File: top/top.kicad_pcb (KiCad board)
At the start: 4 copper layers, 28.3 x 40 mm, 22 parts, among them P1 CONN_10, P2 CONN_5, U1 IQS572, U4 ESD

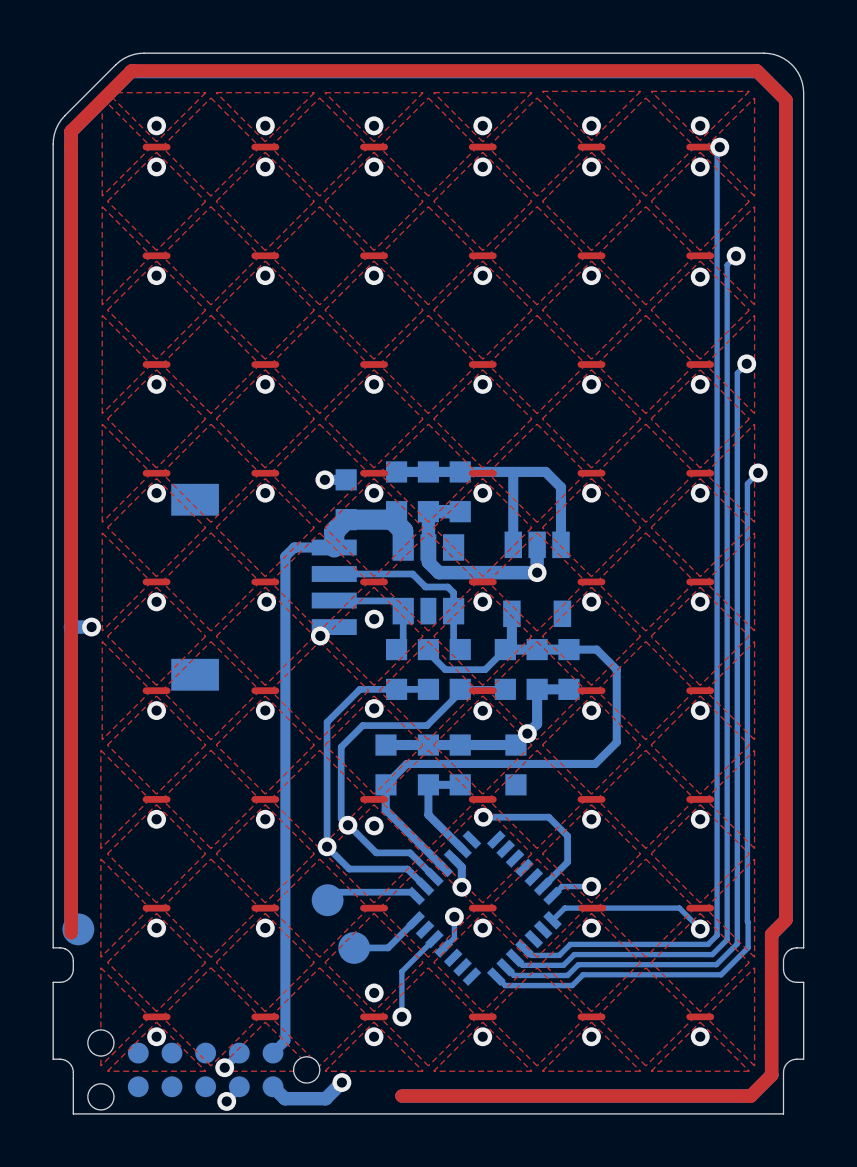
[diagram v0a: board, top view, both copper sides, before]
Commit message: First final modified board.
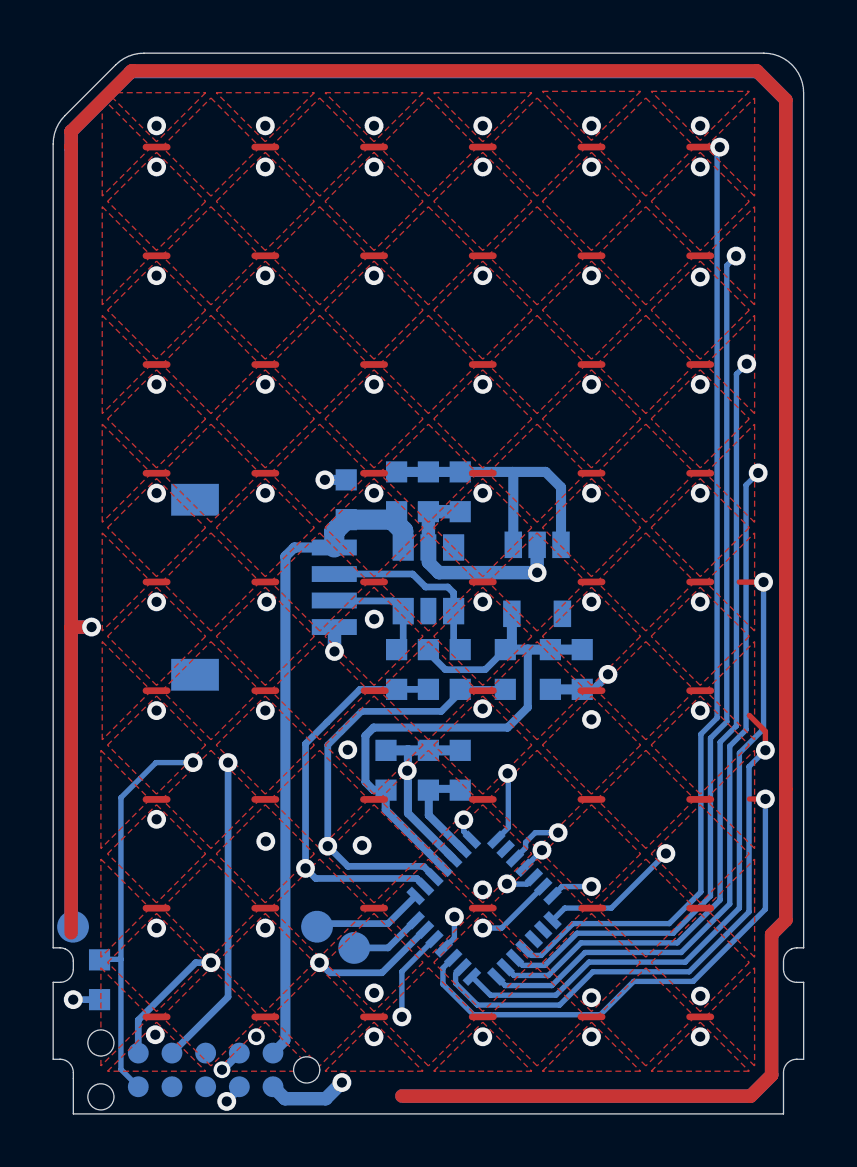
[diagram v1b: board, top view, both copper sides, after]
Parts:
- moved C1 17.7 mm to (193.3, 153.4), turned to 90 degrees
- moved TP_TOUT1 1.08 mm to (201.5, 151.4)
- moved C12 0.50 mm to (210.3, 141.7)
- moved C6 0.50 mm to (211.5, 141.7)
- moved TP_GND1 0.22 mm to (192.3, 151.4)
- moved C3 0.20 mm to (206.9, 145.5)
- moved C4 0.20 mm to (205.7, 145.5)
- moved C5 0.20 mm to (204.1, 145.5)
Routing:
- net (no net): track 41.6 -> 0.00 mm
- net /TX4: track 0.00 -> 30.1 mm, vias 0 -> 1
- net /NRST: track 0.00 -> 27.5 mm, vias 0 -> 2
- net /TX5: track 0.00 -> 26.4 mm, vias 0 -> 1
- net /RDY: track 0.00 -> 26.0 mm, vias 0 -> 2
- net /TX6: track 0.00 -> 25.0 mm, vias 0 -> 1
- net /RX0: track 34.5 -> 52.1 mm, vias 10 -> 11
- net /PGM: track 0.00 -> 13.8 mm, vias 0 -> 2
- net /RX1: track 34.5 -> 46.4 mm, vias 9 -> 11
- net /RX2: track 34.5 -> 43.4 mm, vias 10 -> 11
- net /TX8: track 3.44 -> 8.24 mm
- net /TX7: track 1.36 -> 6.16 mm
- net /TX1: track 34.5 -> 37.9 mm
- net /TX2: track 31.4 -> 34.8 mm
- net /TX3: track 28.3 -> 31.7 mm
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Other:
- rule via_min_size: 0.7112 -> 0.635
